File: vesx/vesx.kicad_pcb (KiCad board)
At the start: 4 copper layers, 100 x 40 mm, 180 parts, among them J1 TYPE-C-31-M-12, J2 Conn_01x05, J3 Conn_01x06, J4 Conn_01x03, J5 Conn_01x04, J6 STLINK, J7 Conn_01x04, J8 CAN, U1 Opamp_Quad, U2 LM1117DT-3.3, U3 LM5164DDA, U4 TO220_replacement_module, U5 L6498DTR, U6 L6498DTR, U7 STM32F405RGTx, U8 L6498DTR, U9 SN65HVD230DR, Y2 8MHz

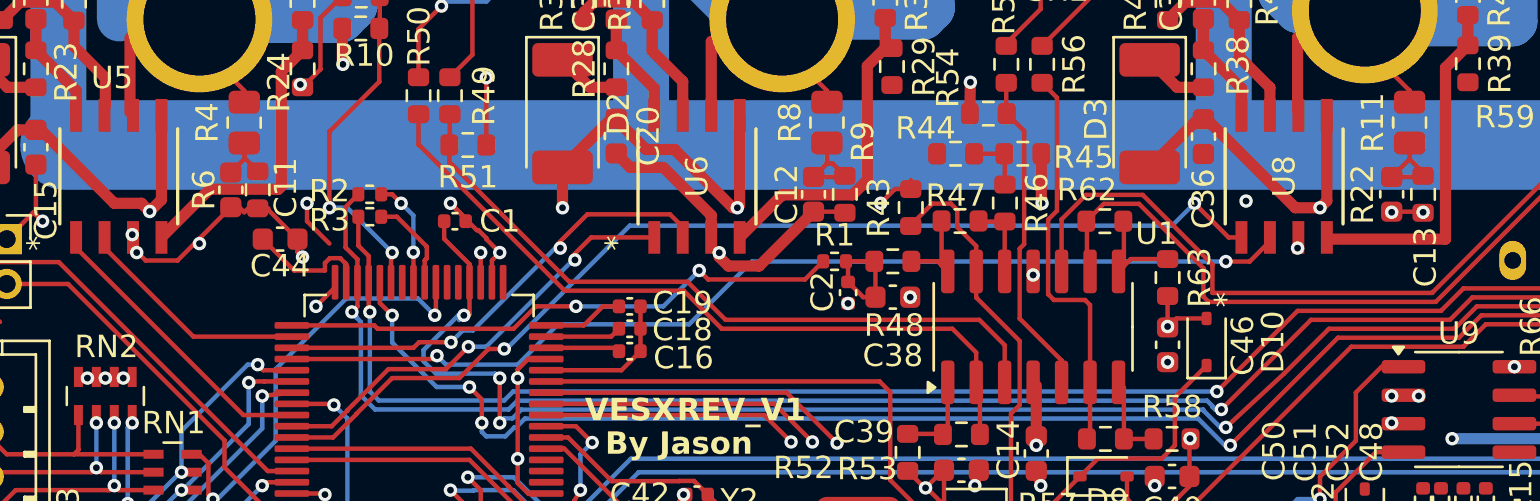
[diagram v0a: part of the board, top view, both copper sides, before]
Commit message: fix
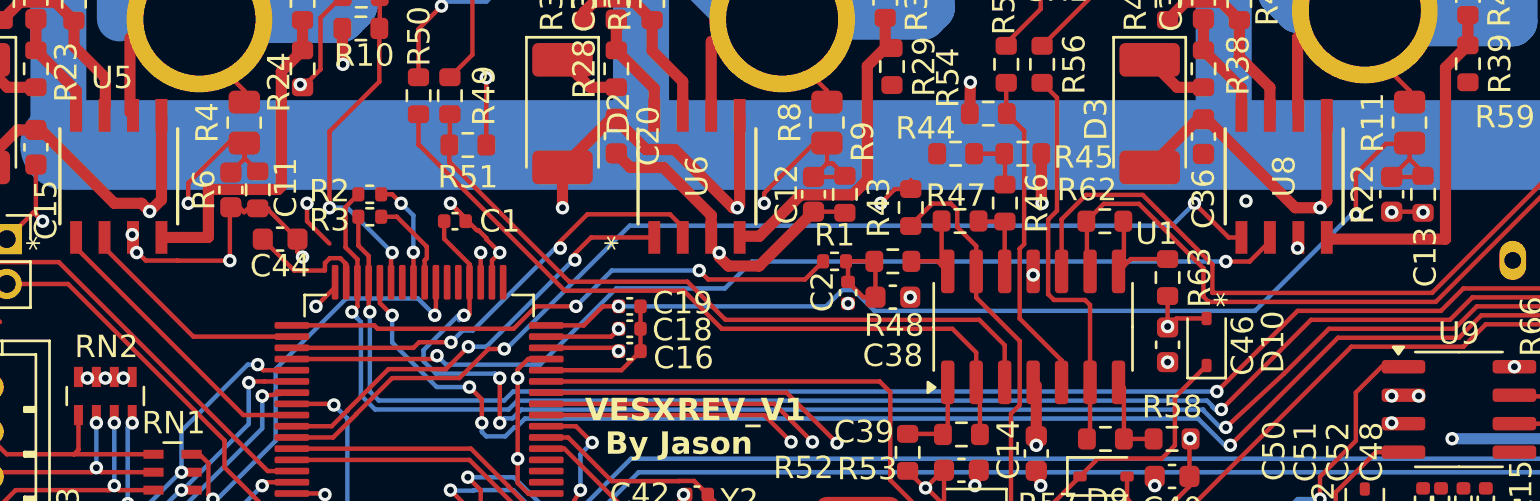
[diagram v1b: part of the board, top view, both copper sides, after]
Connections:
- R11 pad 1: /MCU/VOLTAGE{PHASE} -> PA2
- R4 pad 1: /MCU/VOLTAGE{PHASE} -> PA0
- R8 pad 1: /MCU/VOLTAGE{PHASE} -> PA1
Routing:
- net PA2: track 3.60 -> 43.6 mm, vias 0 -> 2
- net PA0: track 3.31 -> 29.2 mm, vias 0 -> 2
- net PA1: track 3.39 -> 16.2 mm, vias 0 -> 2
- net GND: track 329.6 -> 330.9 mm
- net Net-(U5-LVG): track 14.1 -> 15.3 mm

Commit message: Revert "fix"
This reverts commit 630a2a7c171c78306201b3488f63a123b135c984.
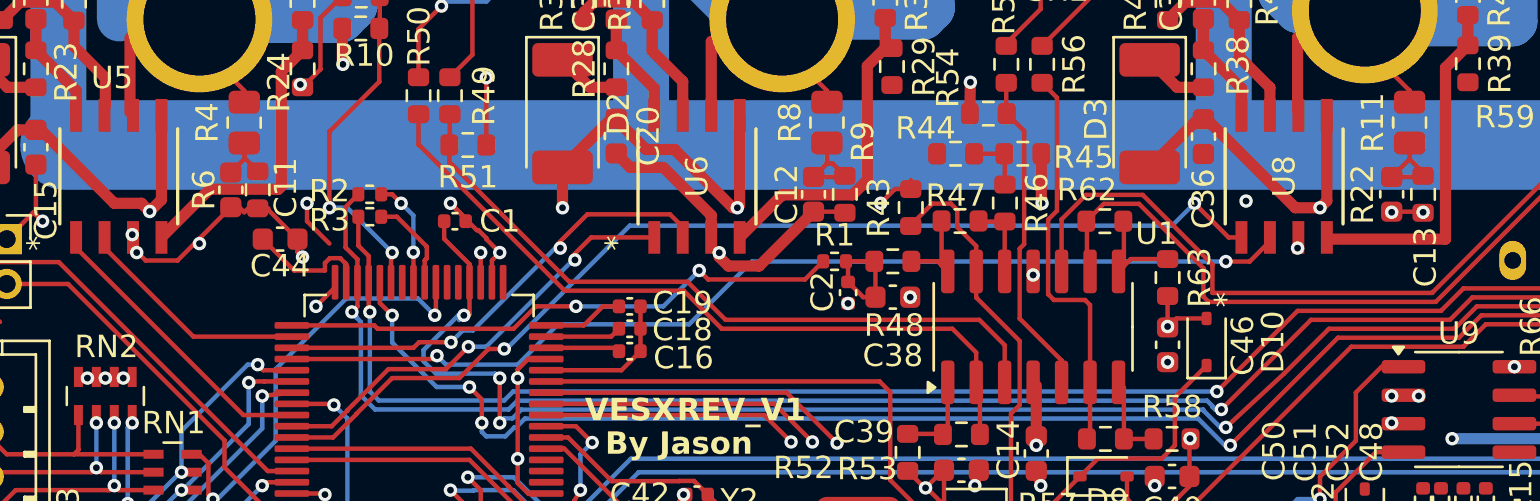
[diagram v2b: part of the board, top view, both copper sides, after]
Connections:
- R11 pad 1: PA2 -> /MCU/VOLTAGE{PHASE}
- R4 pad 1: PA0 -> /MCU/VOLTAGE{PHASE}
- R8 pad 1: PA1 -> /MCU/VOLTAGE{PHASE}
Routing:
- net PA2: track 43.6 -> 3.60 mm, vias 2 -> 0
- net PA0: track 29.2 -> 3.31 mm, vias 2 -> 0
- net PA1: track 16.2 -> 3.39 mm, vias 2 -> 0
- net GND: track 330.9 -> 329.6 mm
- net Net-(U5-LVG): track 15.3 -> 14.1 mm
